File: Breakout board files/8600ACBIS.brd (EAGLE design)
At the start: 22.7 x 17.7 mm, 9 parts, among them IC1 SI8600AC-B-IS

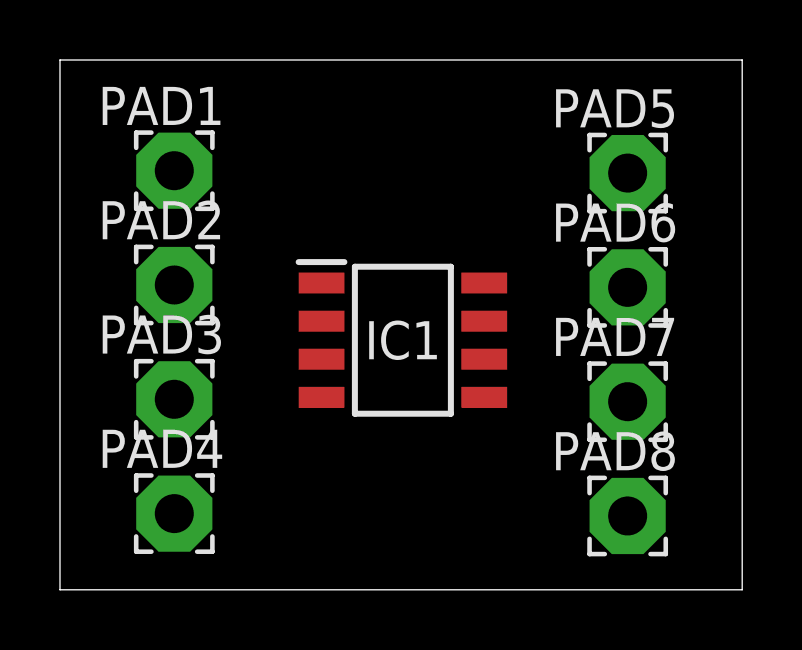
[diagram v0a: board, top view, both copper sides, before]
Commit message: Breakout Board Solutions
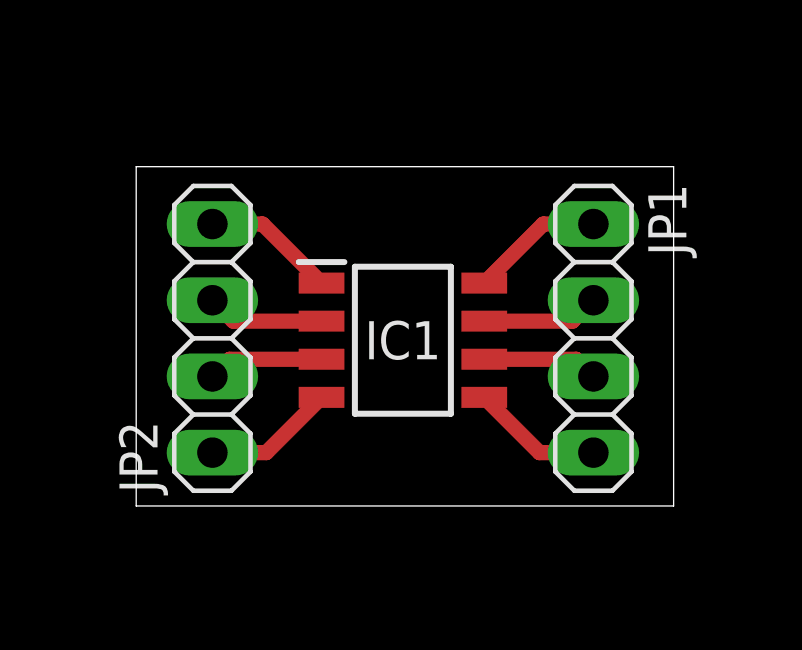
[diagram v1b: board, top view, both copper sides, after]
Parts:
- removed PAD1, PAD2, PAD3, PAD4, PAD5, PAD6, PAD7, PAD8: (no value), ee2parts:2,54/1,1
- added JP1, JP2: (no value), pinhead:1X04
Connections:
- net N$1: now also JP2.4; no longer PAD1.1
- net N$2: now also JP2.3; no longer PAD2.1
- net N$3: now also JP2.2; no longer PAD3.1
- net N$4: now also JP2.1; no longer PAD4.1
- net N$5: now also IC1.8, JP1.1; no longer IC1.5, PAD8.1
- net N$6: now also IC1.7, JP1.2; no longer IC1.6, PAD7.1
- net N$7: now also IC1.6, JP1.3; no longer IC1.7, PAD6.1
- net N$8: now also IC1.5, JP1.4; no longer IC1.8, PAD5.1
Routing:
- net N$5: track 0.00 -> 4.45 mm
- net N$1: track 0.00 -> 4.45 mm
- net N$8: track 0.00 -> 4.40 mm
- net N$4: track 0.00 -> 4.40 mm
- net N$6: track 0.00 -> 3.93 mm
- net N$2: track 0.00 -> 3.93 mm
- net N$7: track 0.00 -> 3.87 mm
- net N$3: track 0.00 -> 3.87 mm
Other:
- board size 22.7 x 17.7 mm -> 17.9 x 11.3 mm
